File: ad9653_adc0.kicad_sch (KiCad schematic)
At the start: 20 parts, among them J201 142-0701-201, J202 142-0701-201, J203 142-0701-201, J204 142-0701-201, U201 AD9653BCPZ-125

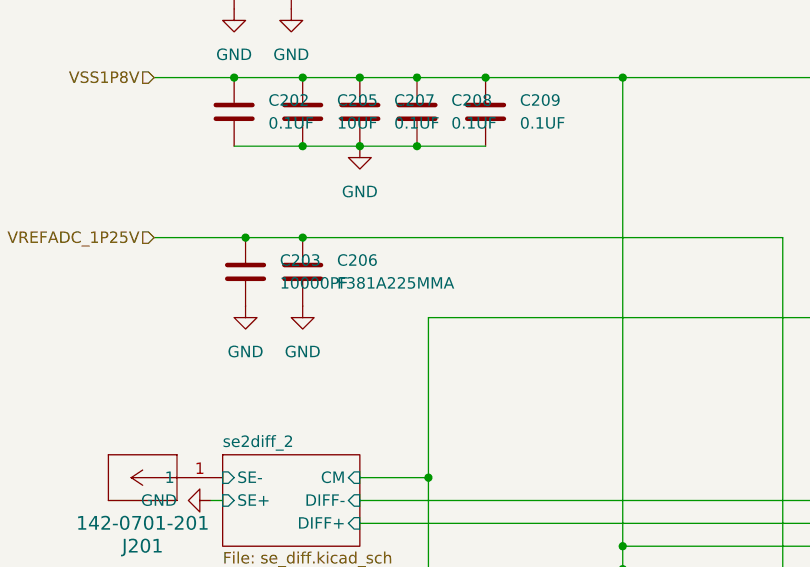
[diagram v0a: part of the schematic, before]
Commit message: value
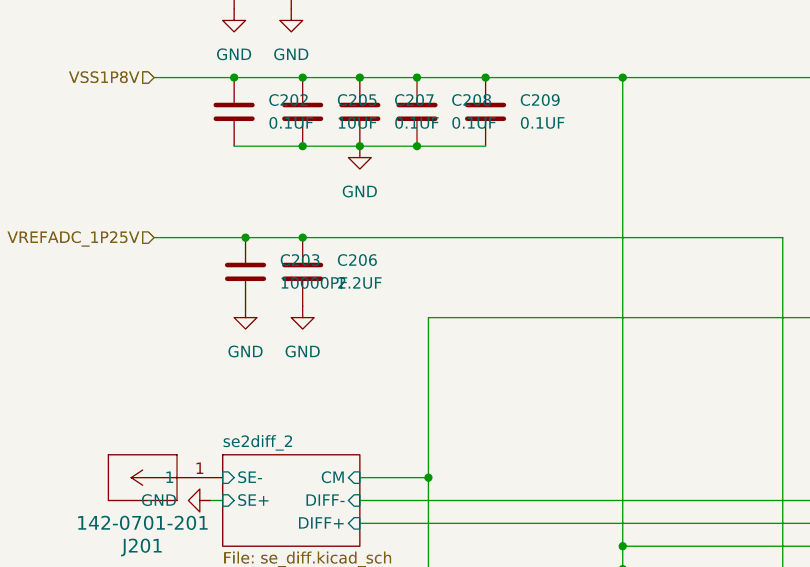
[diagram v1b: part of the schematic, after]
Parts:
- C206: value F381A225MMA -> 2.2UF
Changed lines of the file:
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@@
 			)
 		)
-		(property "Value" "F381A225MMA"
+		(property "Value" "2.2UF"
 			(at 58.42 62.2299 0)
 			(effects
@@
 			)
 		)
-		(property "Description" "Unpolarized capacitor"
+		(property "Description" "Tant_poly"
 			(at 54.61 60.96 0)
 			(effects

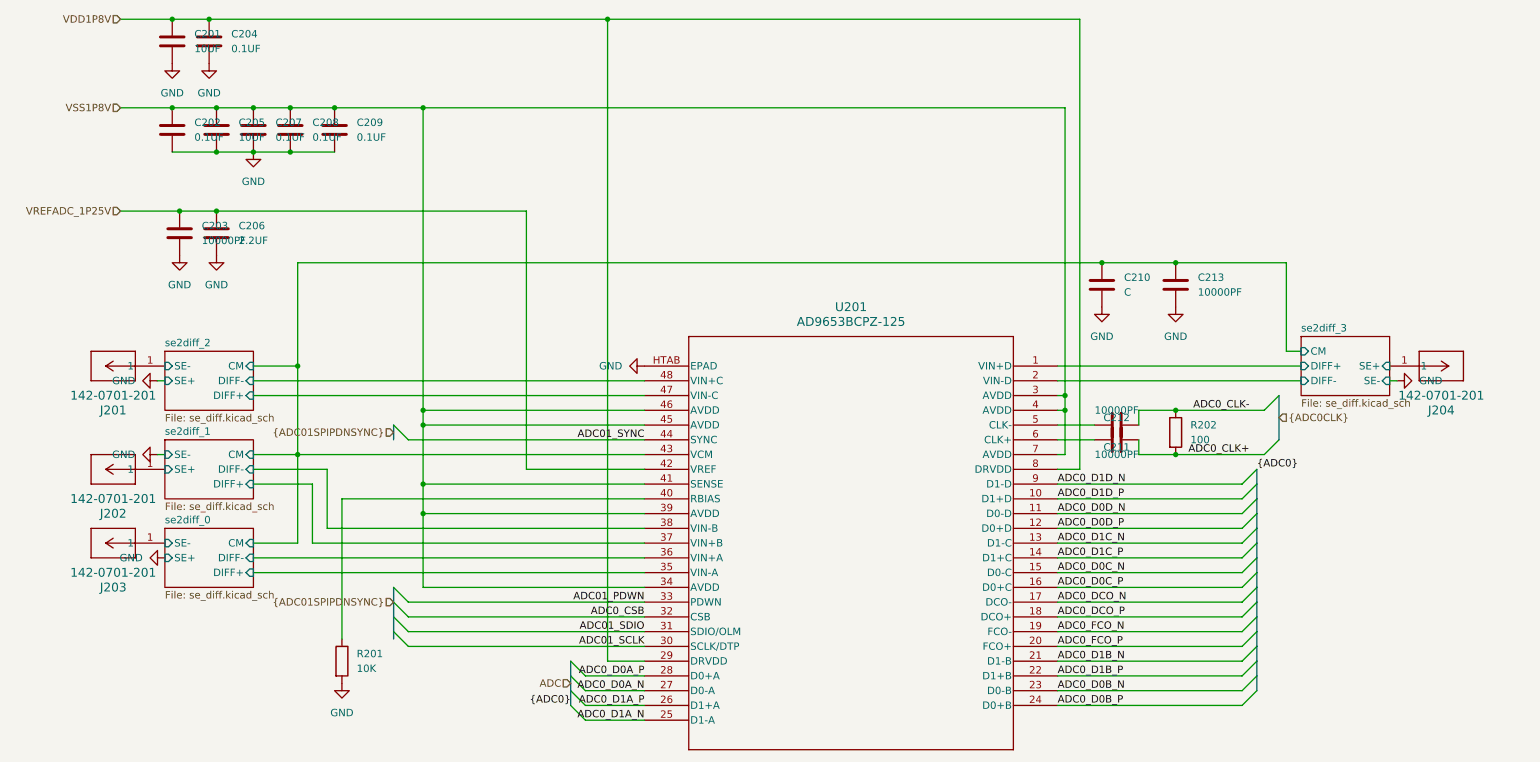
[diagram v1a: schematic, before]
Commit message: lots small updates
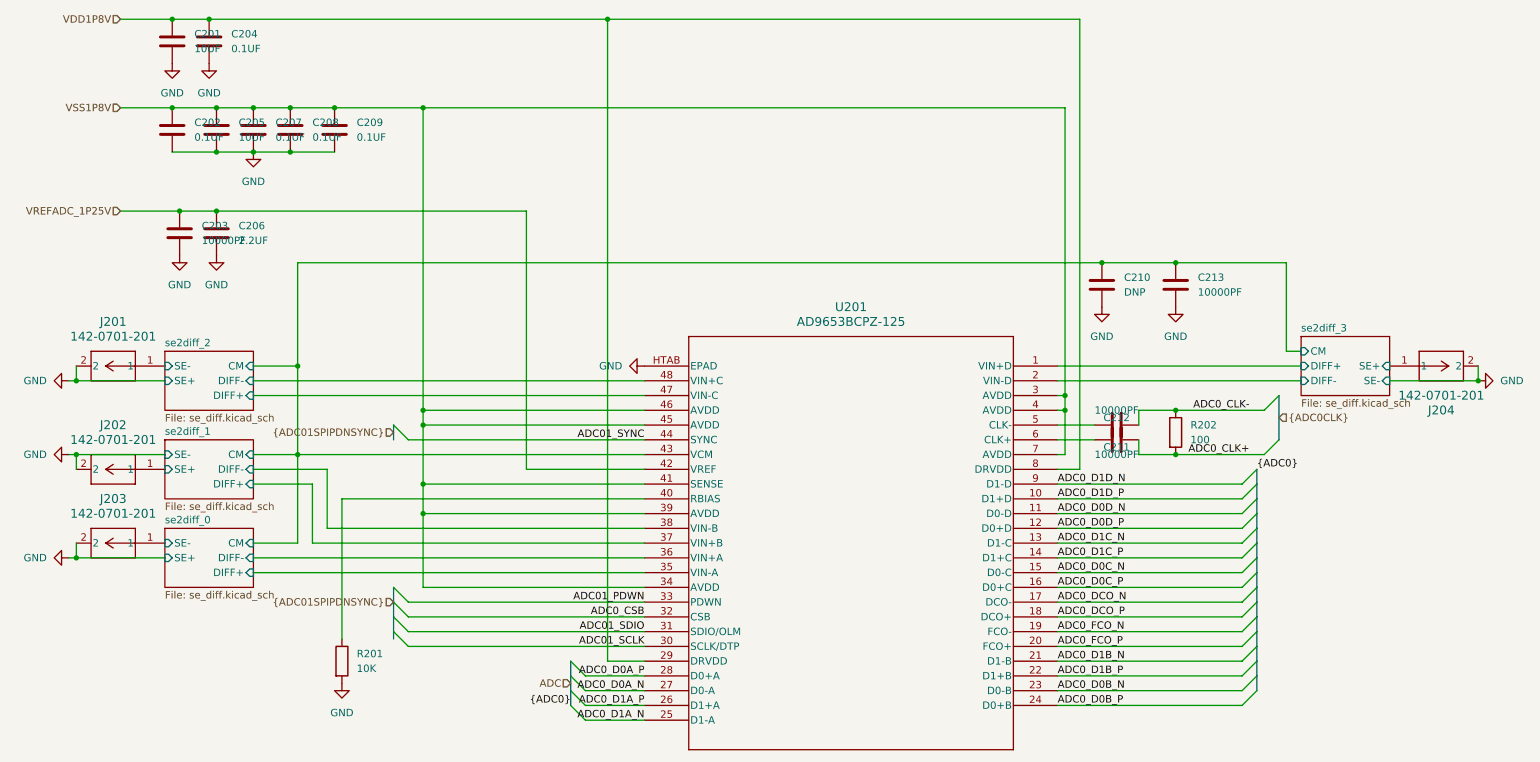
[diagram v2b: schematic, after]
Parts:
- C210: value C -> DNP
- J201, J202, J203, J204: footprint 001_download:CONN_142-0701-201_CIN -> CONN_142-0701-201_CIN; symbol 001_symbol:142-0701-201 -> 001_symbol:142-0701-201_GH
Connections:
- net GND: now also J201.2, J201.3, J201.4, J201.5, J202.2, J202.3, J202.4, J202.5, J203.2, J203.3, J203.4, J203.5, J204.2, J204.3, J204.4, J204.5
